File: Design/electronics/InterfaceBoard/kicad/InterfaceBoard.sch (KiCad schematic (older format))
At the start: 23 parts, among them J1 Screw_Terminal_1x02, J10 Screw_Terminal_1x02, J11 CONN_01X03, J12 Screw_Terminal_1x03, J13 CONN_01X03, J14 CONN_01X03, J2 Screw_Terminal_1x02, J3 Screw_Terminal_1x02, J4 Screw_Terminal_1x02, J5 Screw_Terminal_1x02, J6 Screw_Terminal_1x02, J7 Screw_Terminal_1x02, J8 Screw_Terminal_1x02, J9 Screw_Terminal_1x02

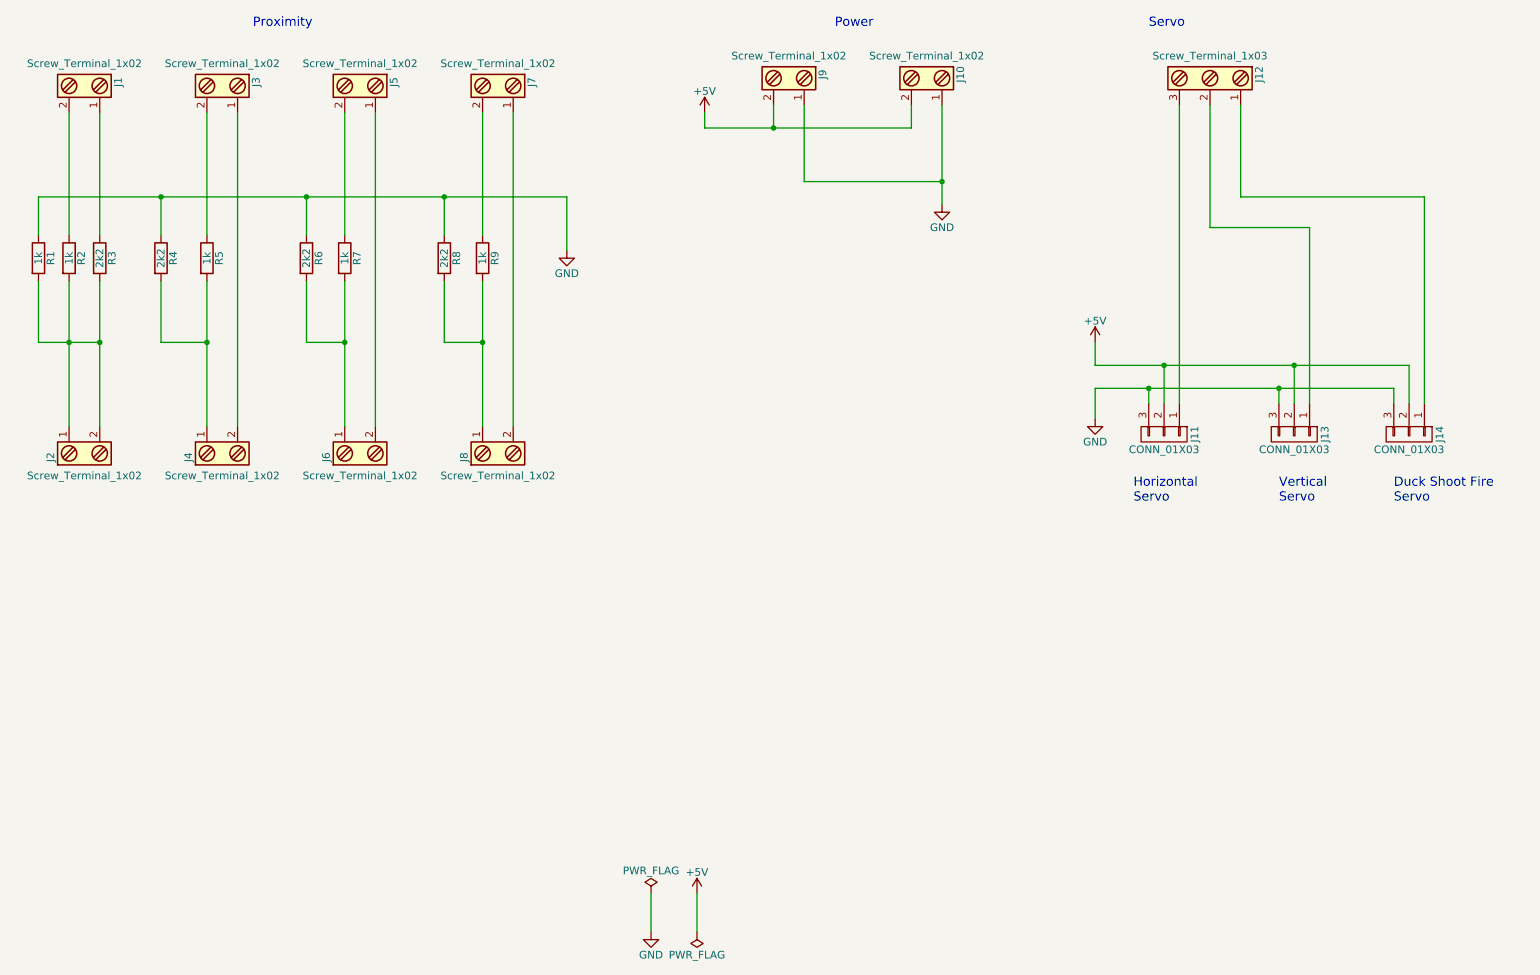
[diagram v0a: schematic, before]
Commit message: updated schematic
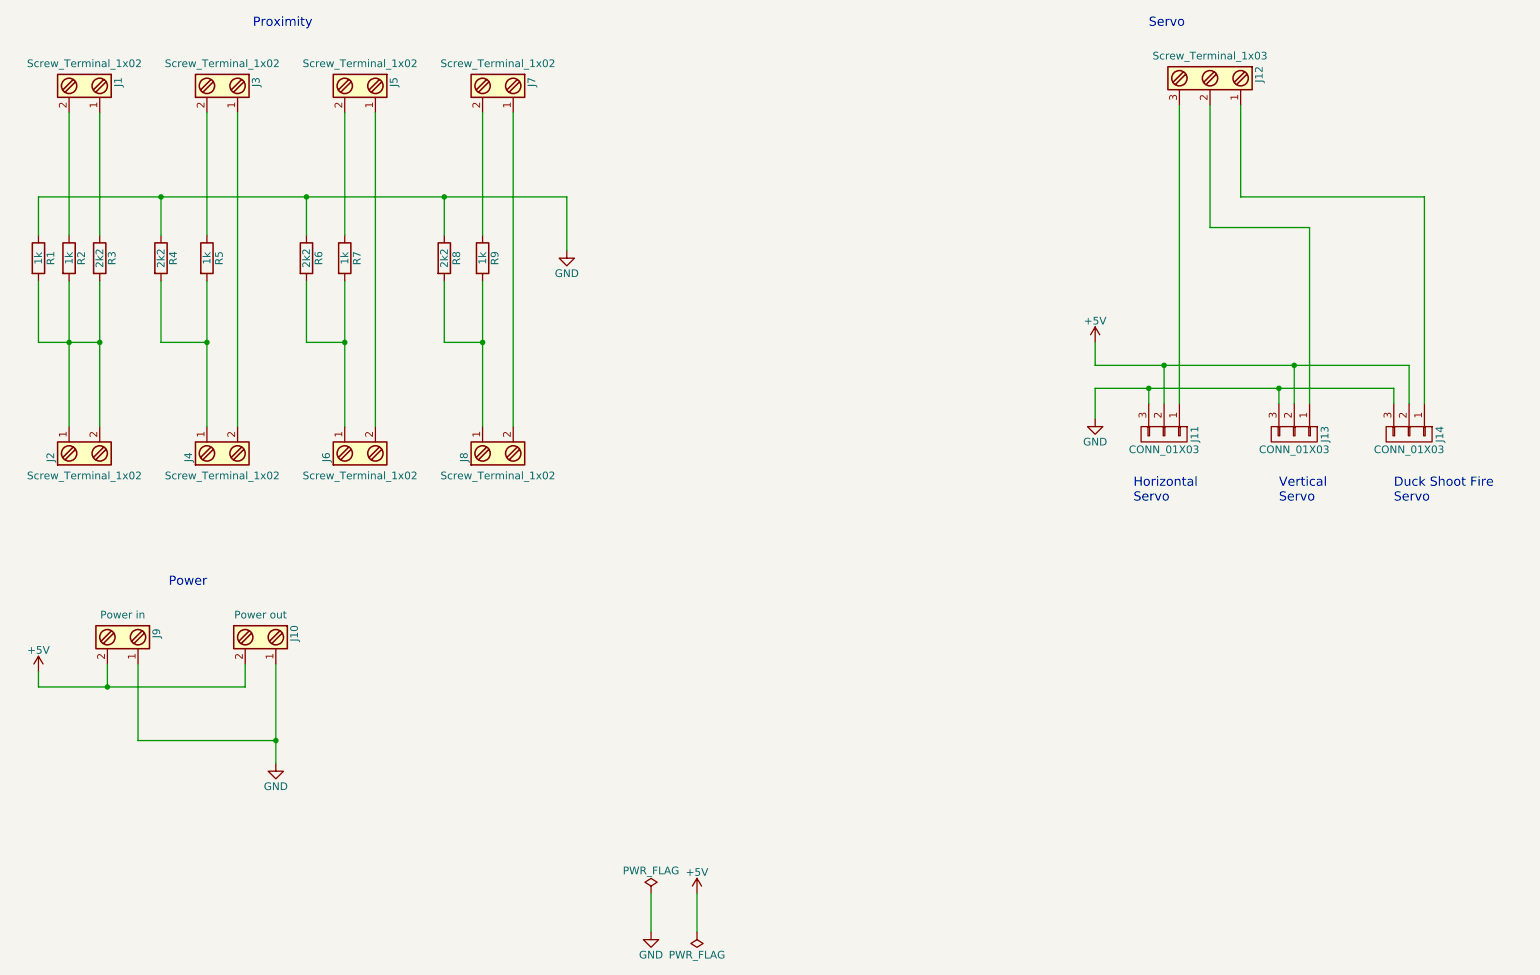
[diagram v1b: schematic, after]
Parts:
- J10: value Screw_Terminal_1x02 -> Power out
- J9: value Screw_Terminal_1x02 -> Power in
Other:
- moved on the sheet: J10, J9
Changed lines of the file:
@@
 L Screw_Terminal_1x02 J10
 U 1 1 5A91D070
-P 7150 1600
-F 0 "J10" H 7150 1850 50  0000 C TNN
-F 1 "Screw_Terminal_1x02" V 7000 1600 50  0000 C TNN
-F 2 "Connectors_Molex:Molex_KK-6410-02_02x2.54mm_Straight" H 7150 1375 50  0001 C CNN
-F 3 "" H 7125 1600 50  0001 C CNN
-	1    7150 1600
+P 2800 5250
+F 0 "J10" H 2800 5500 50  0000 C TNN
+F 1 "Power out" V 2650 5250 50  0000 C TNN
+F 2 "Connectors_Molex:Molex_KK-6410-02_02x2.54mm_Straight" H 2800 5025 50  0001 C CNN
+F 3 "" H 2775 5250 50  0001 C CNN
+	1    2800 5250
 	0    1    1    0
 $EndComp
@@
 Text Notes 2750 1300 0    60   ~ 0
 Proximity
-Text Notes 6550 1300 0    60   ~ 0
+Text Notes 2200 4950 0    60   ~ 0
 Power
 $Comp
 L +5V #PWR05
 U 1 1 5A91D395
-P 5700 1850
-F 0 "#PWR05" H 5700 1700 50  0001 C CNN
-F 1 "+5V" H 5700 1990 50  0000 C CNN
-F 2 "" H 5700 1850 50  0001 C CNN
-F 3 "" H 5700 1850 50  0001 C CNN
-	1    5700 1850
+P 1350 5500
+F 0 "#PWR05" H 1350 5350 50  0001 C CNN
+F 1 "+5V" H 1350 5640 50  0000 C CNN
+F 2 "" H 1350 5500 50  0001 C CNN
+F 3 "" H 1350 5500 50  0001 C CNN
+	1    1350 5500
 	1    0    0    -1
 $EndComp
@@
 L GND #PWR06
 U 1 1 5A91D3C2
-P 7250 2450
-F 0 "#PWR06" H 7250 2200 50  0001 C CNN
-F 1 "GND" H 7250 2300 50  0000 C CNN
-F 2 "" H 7250 2450 50  0001 C CNN
-F 3 "" H 7250 2450 50  0001 C CNN
-	1    7250 2450
-	1    0    0    -1
-$EndComp
-Wire Wire Line
-	7250 1800 7250 2450
+P 2900 6100
+F 0 "#PWR06" H 2900 5850 50  0001 C CNN
+F 1 "GND" H 2900 5950 50  0000 C CNN
+F 2 "" H 2900 6100 50  0001 C CNN
+F 3 "" H 2900 6100 50  0001 C CNN
+	1    2900 6100
+	1    0    0    -1
+$EndComp
+Wire Wire Line
+	2900 5450 2900 6100
 $Comp
 L CONN_01X03 J13
@@
 L Screw_Terminal_1x02 J9
 U 1 1 5A91E5BC
-P 6250 1600
-F 0 "J9" H 6250 1850 50  0000 C TNN
-F 1 "Screw_Terminal_1x02" V 6100 1600 50  0000 C TNN
-F 2 "Connectors_Molex:Molex_KK-6410-02_02x2.54mm_Straight" H 6250 1375 50  0001 C CNN
-F 3 "" H 6225 1600 50  0001 C CNN
-	1    6250 1600
-	0    1    1    0
-$EndComp
-Wire Wire Line
-	5700 1950 7050 1950
-Connection ~ 6150 1950
-Wire Wire Line
-	7050 1950 7050 1800
-Connection ~ 7250 2300
-Wire Wire Line
-	6350 1800 6350 2300
-Wire Wire Line
-	6350 2300 7250 2300
-Wire Wire Line
-	5700 1950 5700 1850
-Wire Wire Line
-	6150 1800 6150 1950
+P 1900 5250
+F 0 "J9" H 1900 5500 50  0000 C TNN
+F 1 "Power in" V 1750 5250 50  0000 C TNN
+F 2 "Connectors_Molex:Molex_KK-6410-02_02x2.54mm_Straight" H 1900 5025 50  0001 C CNN
+F 3 "" H 1875 5250 50  0001 C CNN
+	1    1900 5250
+	0    1    1    0
+$EndComp
+Connection ~ 1800 5600
+Wire Wire Line
+	2700 5600 2700 5450
+Connection ~ 2900 5950
+Wire Wire Line
+	2000 5450 2000 5950
+Wire Wire Line
+	1350 5600 1350 5500
+Wire Wire Line
+	1800 5600 1800 5450
 Wire Wire Line
 	8250 3350 8250 3500
@@
 Wire Wire Line
 	9200 2400 10400 2400
+Wire Wire Line
+	2000 5950 2900 5950
+Wire Wire Line
+	1350 5600 2700 5600
 $EndSCHEMATC
